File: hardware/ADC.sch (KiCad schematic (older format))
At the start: 21 parts, among them J4 691327310016, J5 691327310016

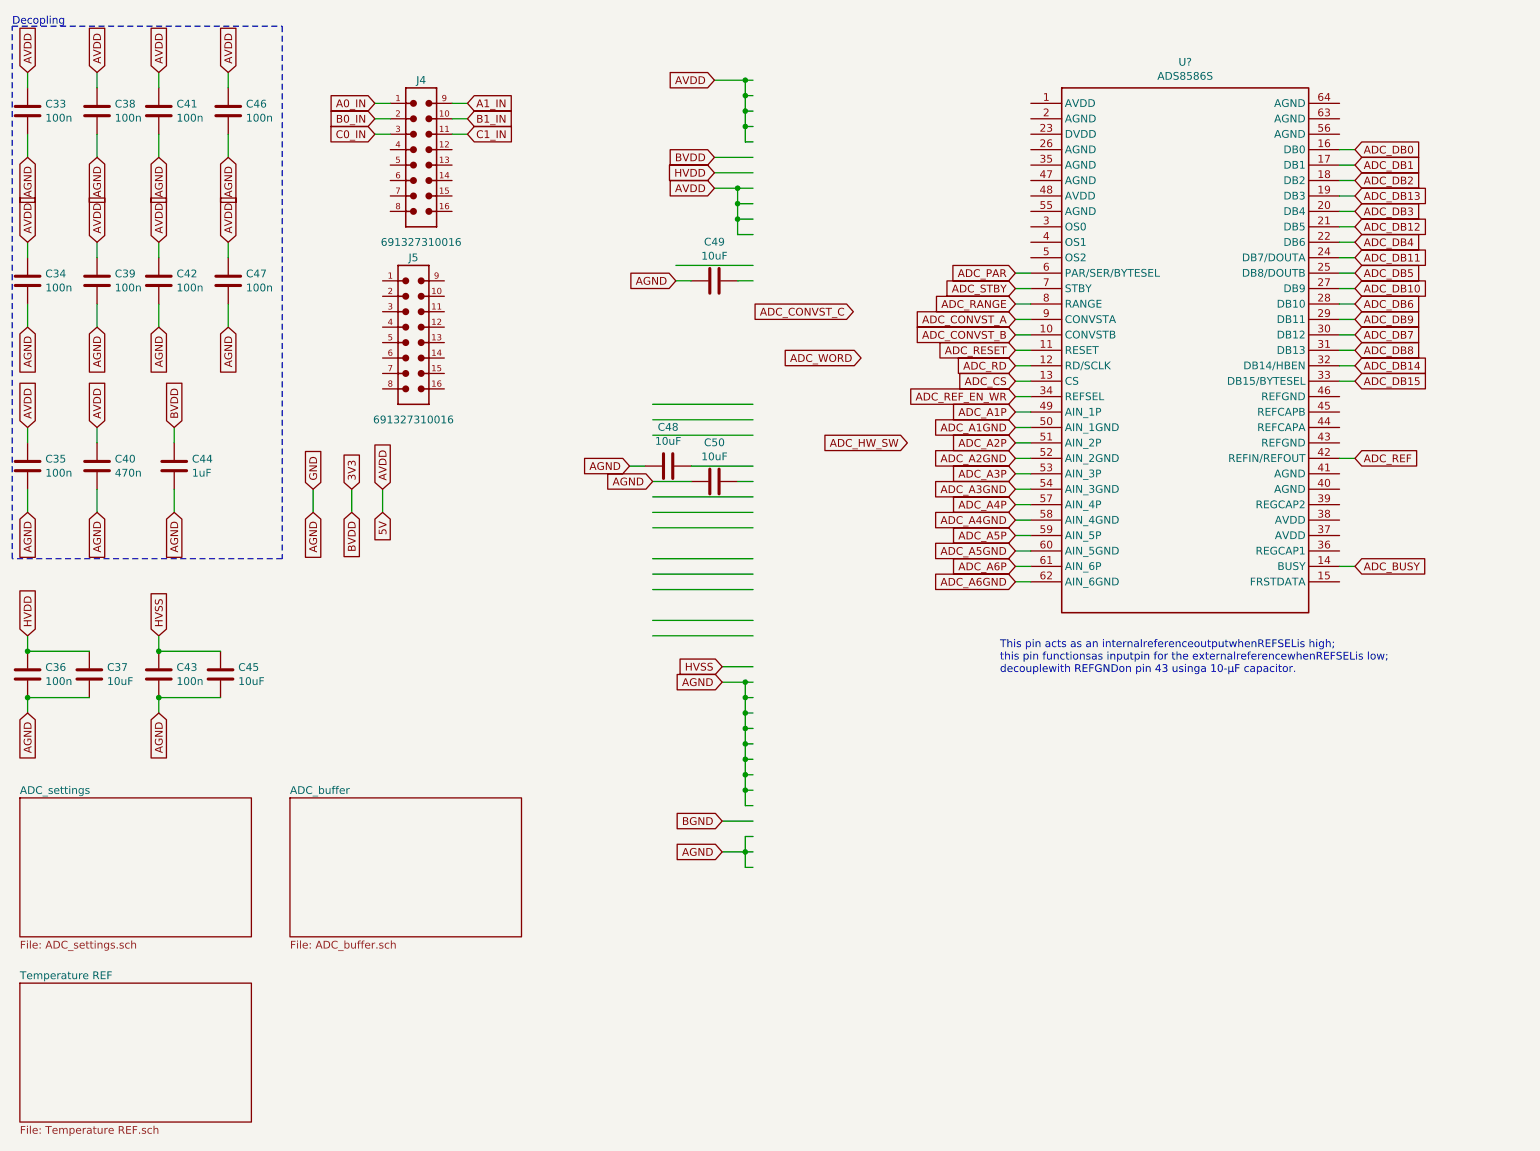
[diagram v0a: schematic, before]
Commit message: Adding last known changes to shematics
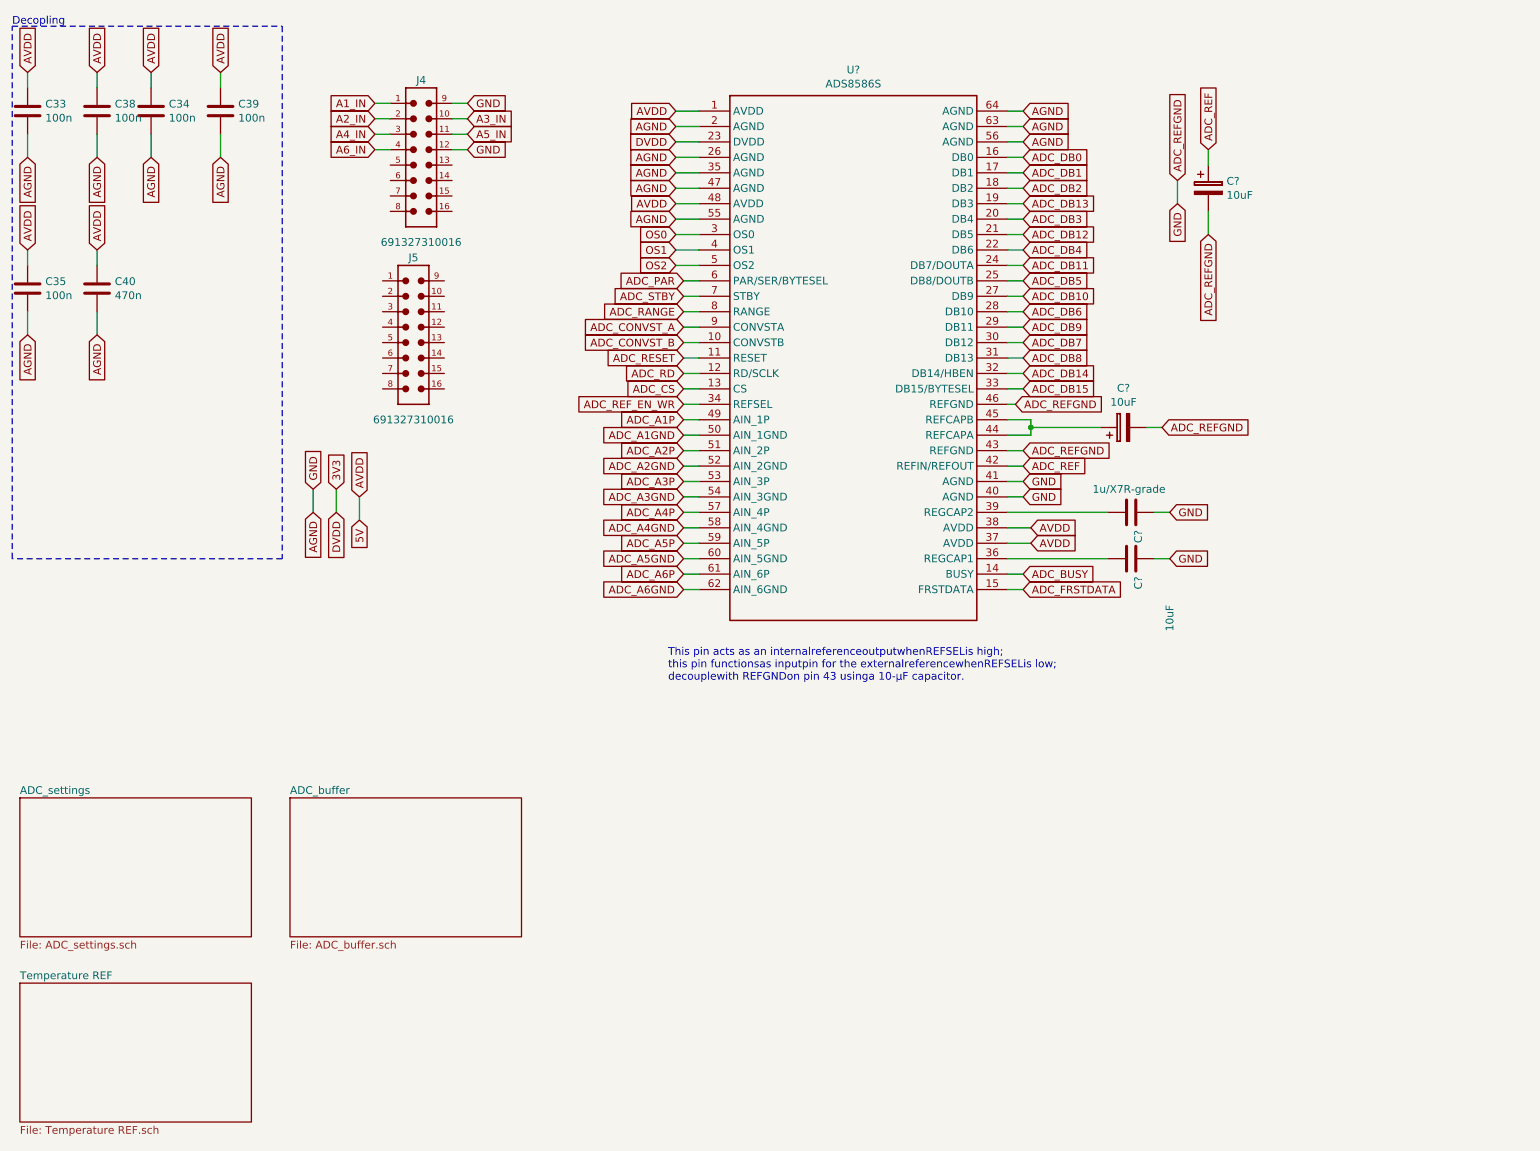
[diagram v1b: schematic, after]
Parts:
- removed C36, C41, C42, C43, C46, C47: 100n, Capacitor_SMD:C_0603_1608Metric, symbol antena:C
- removed C37, C45, C48, C49, C50: 10uF, Capacitor_SMD:C_0603_1608Metric, symbol antena:C
- removed C44: 1uF, Capacitor_SMD:C_0603_1608Metric, symbol antena:C
- added C? (x2): 10uF, symbol antena:CP
- added C?: 10uF, Capacitor_SMD:C_0603_1608Metric, symbol antena:C
- added C?: 1u/X7R-grade, Capacitor_SMD:C_0603_1608Metric, symbol antena:C
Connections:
- net labels added: A2_IN, A3_IN, A4_IN, A5_IN, A6_IN, ADC_FRSTDATA, ADC_REFGND, DVDD, OS0, OS1, OS2
- net labels removed: A0_IN, ADC_CONVST_C, ADC_HW_SW, ADC_WORD, B0_IN, B1_IN, BGND, BVDD, C0_IN, C1_IN, HVDD, HVSS
- wire segments 142 -> 96
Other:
- moved on the sheet: C34, C35, C39, C40, U?
